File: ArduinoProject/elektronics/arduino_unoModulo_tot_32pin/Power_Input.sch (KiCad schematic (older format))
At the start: 8 parts, among them IC401 MC33269ST-5.OT3, U402 LP2985-3.3, X2 DG3XX-02-3.5

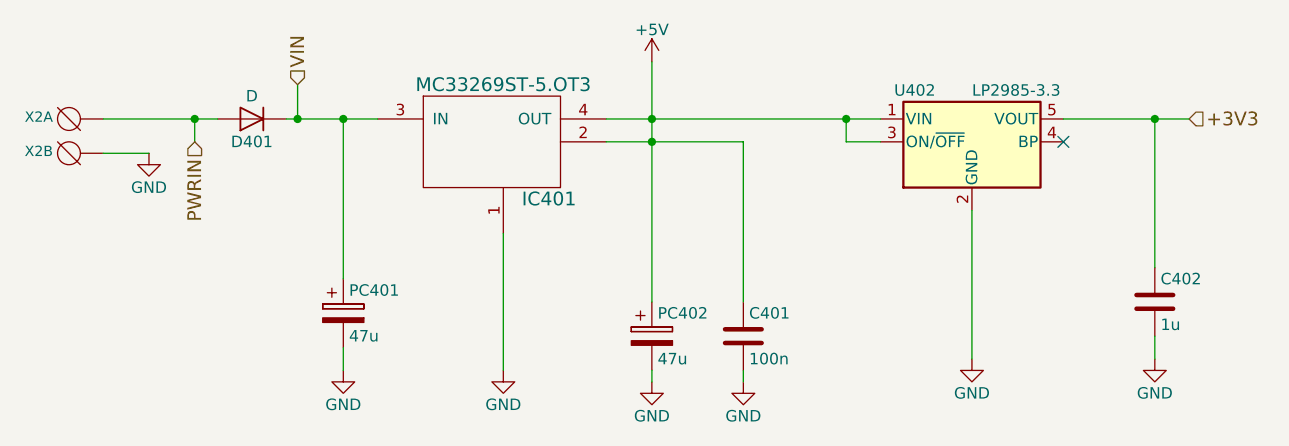
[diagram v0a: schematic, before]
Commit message: new components2
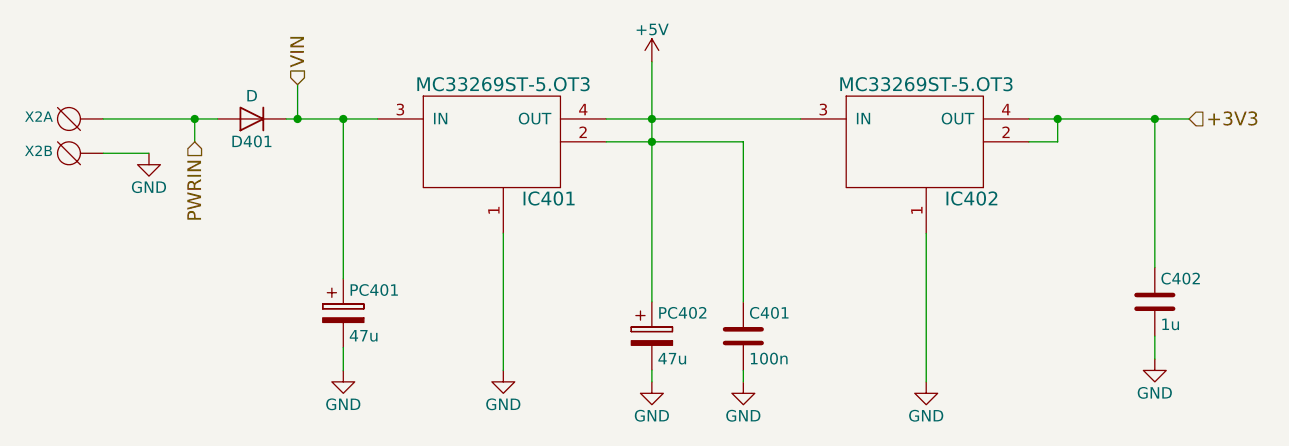
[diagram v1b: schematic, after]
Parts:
- removed U402: LP2985-3.3, TO_SOT_Packages_SMD:SOT-23-5, symbol LP2985-3.3
- added IC402: MC33269ST-5.OT3, PHT6NQ10T_135:SOT230P700X180-4N, symbol MC33269ST-5.OT3
- D401: footprint Diodes_SMD:D_0805 -> Diodes_SMD:D_MicroMELF_Hadsoldering
- IC401: footprint MC33269ST-3.3T3G:SOT230P700X175-4N -> PHT6NQ10T_135:SOT230P700X180-4N
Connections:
- net +3V3: now also IC402.2, IC402.4 (OUT)
- net +5V: now also IC402.3 (IN)
- net GND: now also IC402.1
- no-connect marks 1 -> 0
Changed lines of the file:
@@
 $EndDescr
-$Comp
-L LP2985-3.3 U402
-U 1 1 5A9664D2
-P 7450 2900
-F 0 "U402" H 7200 3125 50  0000 C CNN
-F 1 "LP2985-3.3" H 7450 3125 50  0000 L CNN
-F 2 "TO_SOT_Packages_SMD:SOT-23-5" H 7450 3225 50  0001 C CNN
-F 3 "" H 7450 2900 50  0001 C CNN
-	1    7450 2900
-	1    0    0    -1
-$EndComp
 $Comp
 L MC33269ST-5.OT3 IC401
@@
 F 0 "IC401" H 5600 2650 60  0000 C CNN
 F 1 "MC33269ST-5.OT3" H 5400 3150 60  0000 C CNN
-F 2 "MC33269ST-3.3T3G:SOT230P700X175-4N" H 5050 2800 60  0001 C CNN
+F 2 "PHT6NQ10T_135:SOT230P700X180-4N" H 5050 2800 60  0001 C CNN
 F 3 "" H 5050 2800 60  0001 C CNN
 	1    5400 2900
@@
 F 0 "D401" H 4300 2900 50  0000 C CNN
 F 1 "D" H 4300 2700 50  0000 C CNN
-F 2 "Diodes_SMD:D_0805" H 4300 2800 50  0001 C CNN
+F 2 "Diodes_SMD:D_MicroMELF_Hadsoldering" H 4300 2800 50  0001 C CNN
 F 3 "" H 4300 2800 50  0001 C CNN
 	1    4300 2800
@@
 Wire Wire Line
 	5400 3900 5400 3300
-Wire Wire Line
-	7050 2800 5850 2800
 Connection ~ 6050 2800
 Wire Wire Line
-	7050 2900 6900 2900
-Wire Wire Line
-	6900 2900 6900 2800
-Connection ~ 6900 2800
-Wire Wire Line
-	7850 2800 8400 2800
+	7700 2800 8400 2800
 Wire Wire Line
 	8250 2800 8250 3450
@@
 L GND #PWR019
 U 1 1 5A97100A
-P 7450 3850
-F 0 "#PWR019" H 7450 3600 50  0001 C CNN
-F 1 "GND" H 7450 3700 50  0000 C CNN
-F 2 "" H 7450 3850 50  0001 C CNN
-F 3 "" H 7450 3850 50  0001 C CNN
-	1    7450 3850
-	1    0    0    -1
-$EndComp
-Wire Wire Line
-	7450 3850 7450 3200
+P 7250 3950
+F 0 "#PWR019" H 7250 3700 50  0001 C CNN
+F 1 "GND" H 7250 3800 50  0000 C CNN
+F 2 "" H 7250 3950 50  0001 C CNN
+F 3 "" H 7250 3950 50  0001 C CNN
+	1    7250 3950
+	1    0    0    -1
+$EndComp
+Wire Wire Line
+	7250 3950 7250 3300
 Wire Wire Line
 	5850 2900 6450 2900
@@
 Wire Wire Line
 	6050 3950 6050 3900
-NoConn ~ 7850 2900
 Connection ~ 8250 2800
 Text HLabel 8400 2800 2    60   Input ~ 0
@@
 	-1   0    0    1
 $EndComp
+$Comp
+L MC33269ST-5.OT3 IC402
+U 1 1 5AA92A2E
+P 7250 2900
+F 0 "IC402" H 7450 2650 60  0000 C CNN
+F 1 "MC33269ST-5.OT3" H 7250 3150 60  0000 C CNN
+F 2 "PHT6NQ10T_135:SOT230P700X180-4N" H 6900 2800 60  0001 C CNN
+F 3 "" H 6900 2800 60  0001 C CNN
+	1    7250 2900
+	1    0    0    -1
+$EndComp
+Wire Wire Line
+	5850 2800 6700 2800
+Wire Wire Line
+	7700 2900 7825 2900
+Wire Wire Line
+	7825 2900 7825 2800
+Connection ~ 7825 2800
 $EndSCHEMATC
